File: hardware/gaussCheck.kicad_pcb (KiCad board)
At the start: 2 copper layers, 27.8 x 91.7 mm, 42 parts, among them J1 USB_C_Receptacle_USB2.0, J2 SWD, SW1 PTS810, SW2 CK KSC2, SW3 CK KSC2, SW4 CK KSC2, U1 TLV493D, U2 VIM-878-DP, U3 ATSAML22N18A-AUT, U4 TPS613221ADBV, Y1 32.768kHz

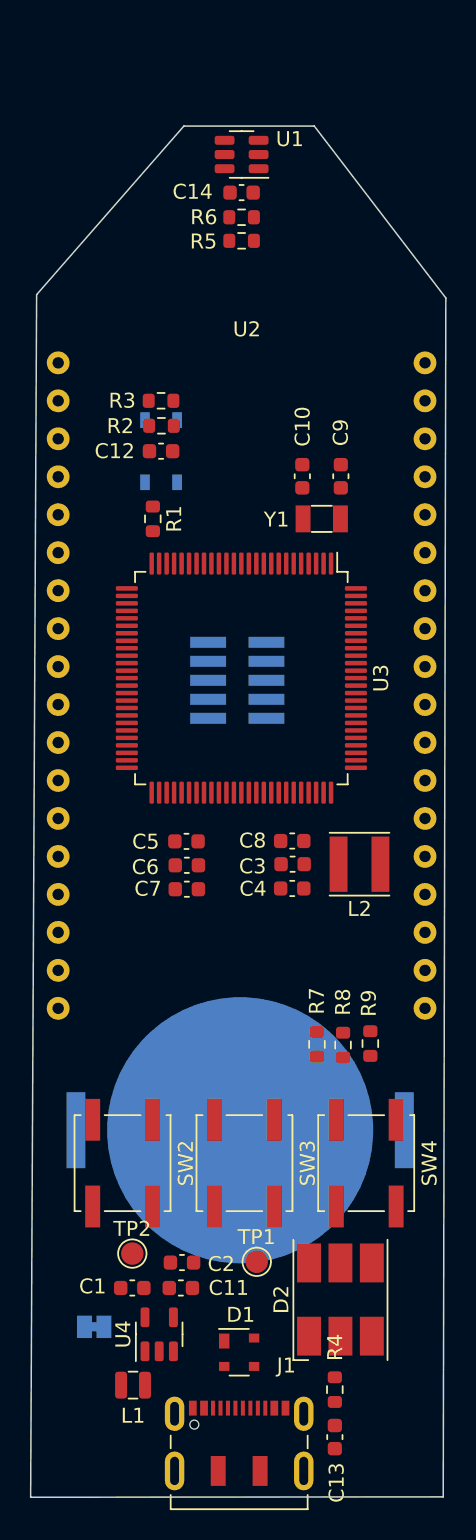
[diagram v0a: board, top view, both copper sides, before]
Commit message: continue
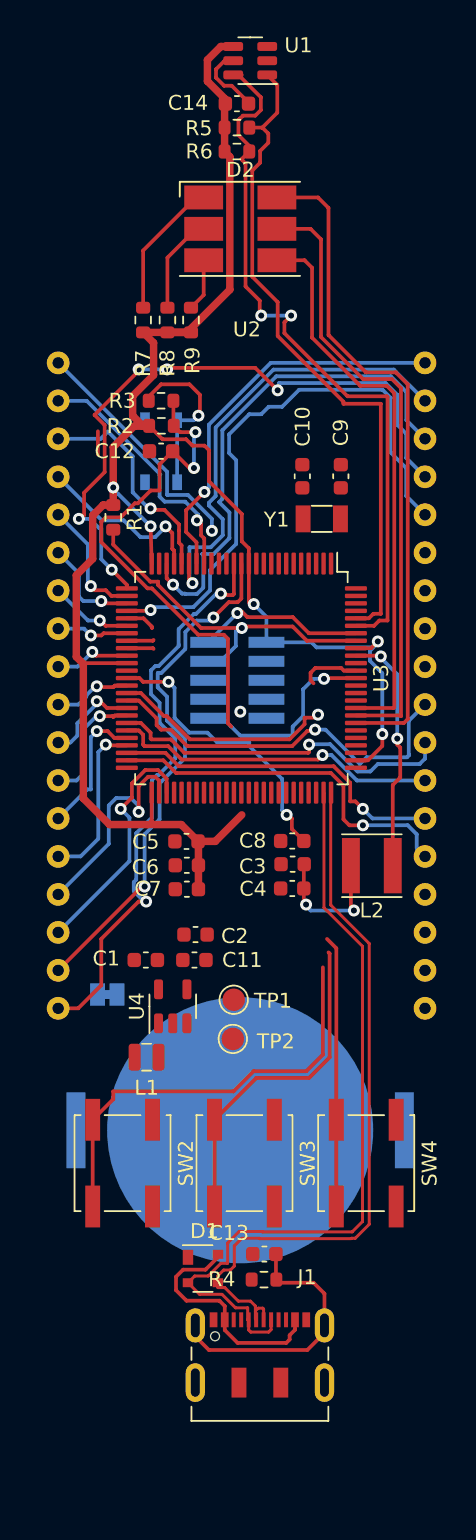
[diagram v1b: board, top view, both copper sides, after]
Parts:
- moved D2 71.9 mm to (141.5, 64.1), turned to 0 degrees
- moved R8 49.9 mm to (136.6, 70.2), turned to 90 degrees
- moved R9 49.9 mm to (138.2, 70.2), turned to 90 degrees
- moved R7 49.8 mm to (135.0, 70.2), turned to 90 degrees
- moved JP1 22.2 mm to (132.6, 115.3)
- moved U4 22.0 mm to (137.0, 116.1)
- moved C2 22.0 mm to (138.5, 111.3)
- moved C1 22.0 mm to (135.2, 113.0)
- moved C11 22.0 mm to (138.4, 113.0)
- moved L1 22.0 mm to (135.2, 119.5)
- moved TP1 17.6 mm to (141.1, 115.7)
- moved TP2 15.9 mm to (141.0, 118.3)
- moved C13 13.1 mm to (143.1, 132.7), turned to 180 degrees
- moved R4 8.75 mm to (143.1, 134.4), turned to 180 degrees
- moved R5 7.58 mm to (141.3, 57.3)
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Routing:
- net +3V3: track 0.00 -> 129.2 mm, vias 0 -> 5
- net /MCU/D-: track 0.00 -> 52.5 mm
- net /MCU/SDA: track 0.00 -> 49.1 mm, vias 0 -> 2
- net /MCU/D+: track 0.00 -> 48.5 mm
- net /MCU/~{RESET}: track 0.00 -> 47.8 mm, vias 0 -> 4
- net /MCU/SCL: track 0.00 -> 45.0 mm
- net /MCU/LED1: track 0.00 -> 44.9 mm
- net /MCU/DPCBA2: track 0.00 -> 44.7 mm, vias 0 -> 5
- net /MCU/LED2: track 0.00 -> 41.5 mm
- net /MCU/MNGH3: track 0.00 -> 40.2 mm, vias 0 -> 1
- net /MCU/COM1: track 0.00 -> 39.1 mm, vias 0 -> 2
- net /MCU/LED3: track 0.00 -> 37.9 mm
- net /MCU/COM0: track 0.00 -> 35.0 mm, vias 0 -> 2
- net /MCU/MNGH2: track 0.00 -> 34.1 mm, vias 0 -> 1
- net /MCU/DPCBA1: track 0.00 -> 30.7 mm, vias 0 -> 1
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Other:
- board outline removed
